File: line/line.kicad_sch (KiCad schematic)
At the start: 43 parts, among them J1 MAINS, J2 PWM, Q1 WMM38N60C2, Q2 WMM38N60C2, U1 LM324, U2 LTV-817S

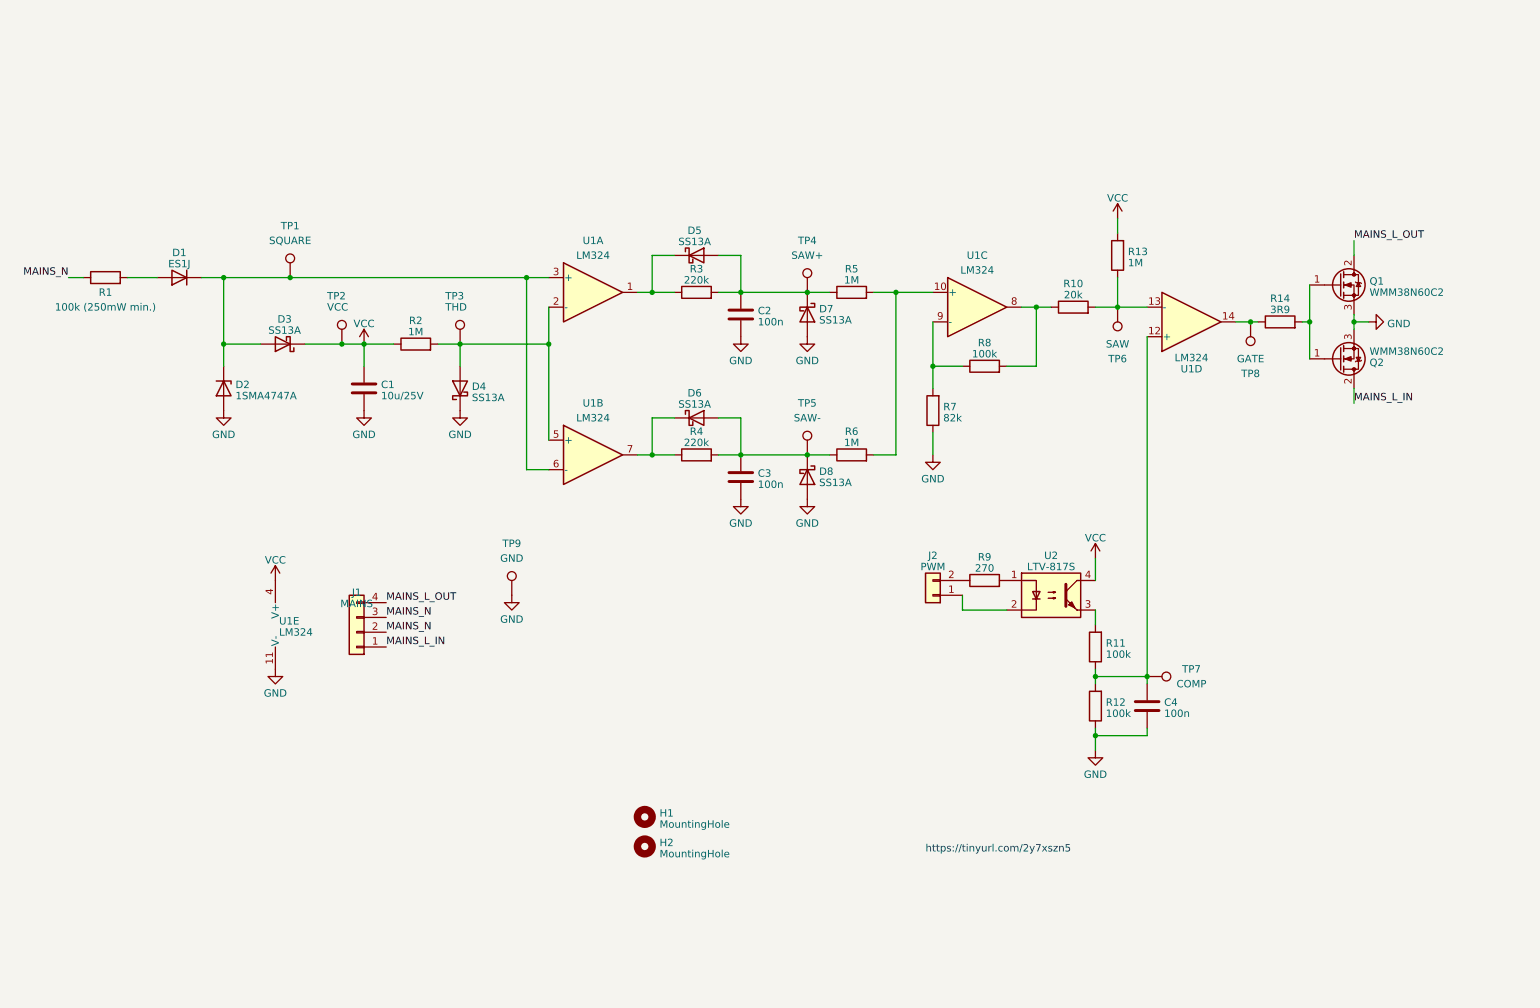
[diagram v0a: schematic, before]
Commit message: WIP
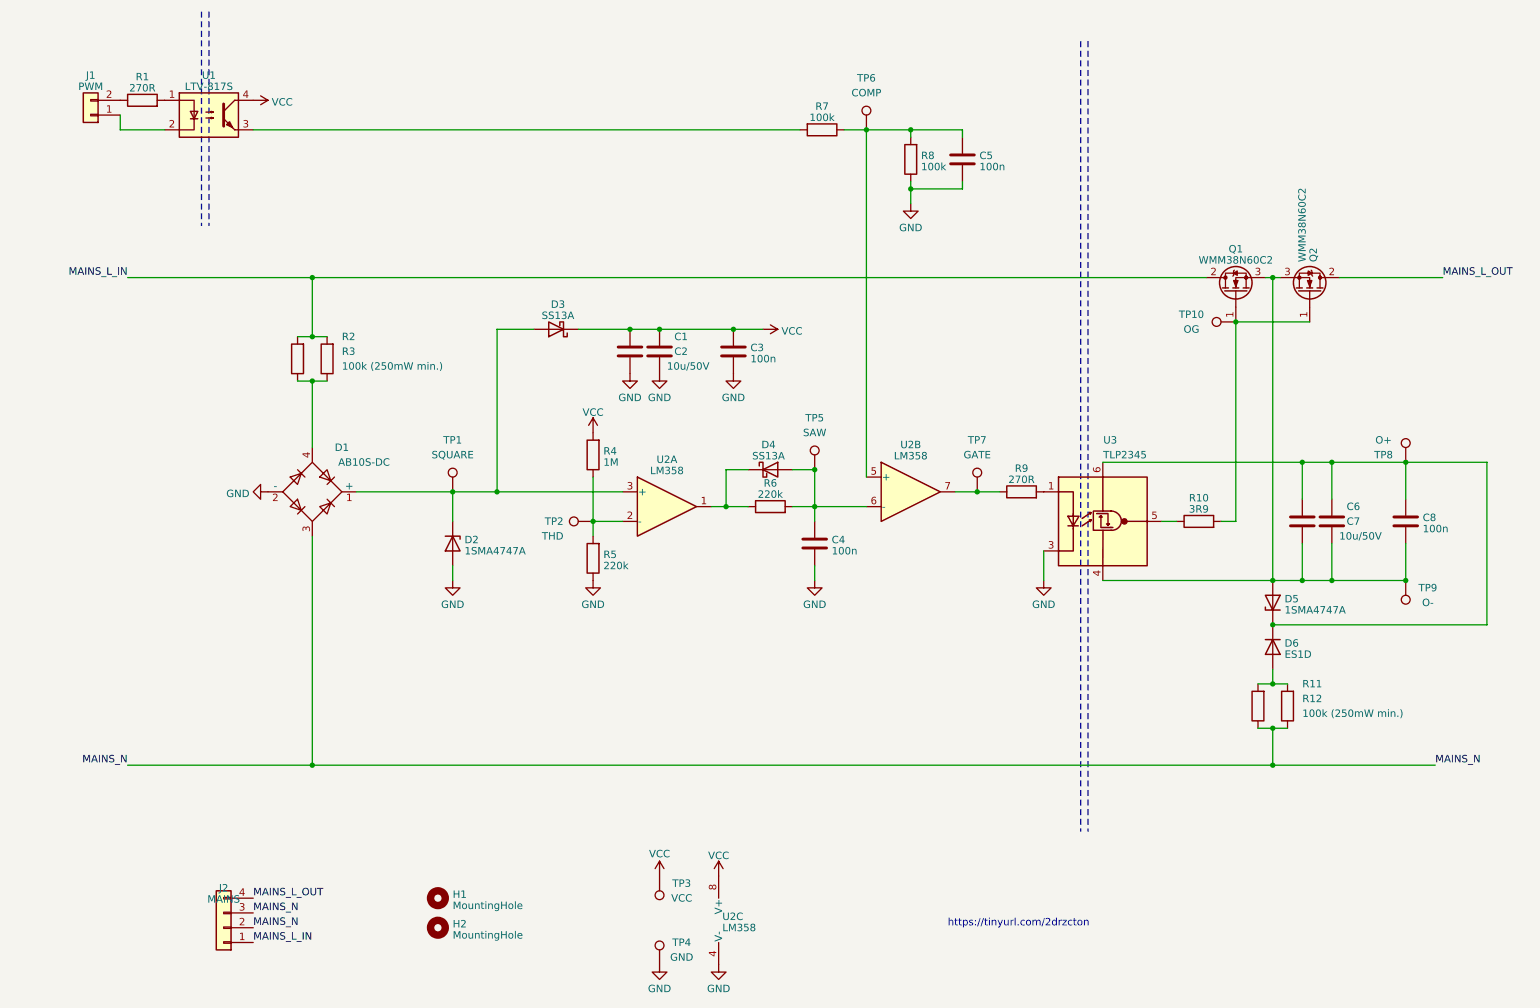
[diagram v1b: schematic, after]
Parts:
- removed D1: ES1J, Diode_SMD:D_SMA_Handsoldering, symbol Device:D
- removed D4, D6, D7, D8: SS13A, Diode_SMD:D_SMA_Handsoldering, symbol Device:D_Schottky
- removed R1: 100k (250mW min.), Resistor_SMD:R_1206_3216Metric_Pad1.30x1.75mm_HandSolder, symbol Device:R
- removed R10: 20k, Resistor_SMD:R_0805_2012Metric_Pad1.20x1.40mm_HandSolder, symbol Device:R
- removed R13, R6: 1M, Resistor_SMD:R_0805_2012Metric_Pad1.20x1.40mm_HandSolder, symbol Device:R
- removed R4: 220k, Resistor_SMD:R_0805_2012Metric_Pad1.20x1.40mm_HandSolder, symbol Device:R
- removed R7: 82k, Resistor_SMD:R_0805_2012Metric_Pad1.20x1.40mm_HandSolder, symbol Device:R
- removed R8: 100k, Resistor_SMD:R_0805_2012Metric_Pad1.20x1.40mm_HandSolder, symbol Device:R
- removed TP4: SAW+, TestPoint:TestPoint_Pad_D2.0mm, symbol Connector:TestPoint
- removed TP5: SAW-, TestPoint:TestPoint_Pad_D2.0mm, symbol Connector:TestPoint
- removed U1: LM324, Package_SO:SOIC-14_3.9x8.7mm_P1.27mm, symbol Amplifier_Operational:LM324
- added C2, C6, C7: 10u/50V, Capacitor_SMD:C_1206_3216Metric_Pad1.33x1.80mm_HandSolder, symbol Device:C
- added C8: 100n, Capacitor_SMD:C_0805_2012Metric_Pad1.18x1.45mm_HandSolder, symbol Device:C
- added D1: AB10S-DC, Diode_SMD:Diode_Bridge_Diotec_ABS, symbol Diode_Bridge:ABS10
- added D5: 1SMA4747A, Diode_SMD:D_SMA, symbol Device:D_Zener
- added D6: ES1D, Diode_SMD:D_SMA, symbol Diode:US1D
- added R11, R12, R2, R3: 100k (250mW min.), Resistor_SMD:R_1206_3216Metric_Pad1.30x1.75mm_HandSolder, symbol Device:R
- added R9: 270R, Resistor_SMD:R_0805_2012Metric_Pad1.20x1.40mm_HandSolder, symbol Device:R
- added TP10: OG, TestPoint:TestPoint_Pad_D2.0mm, symbol Connector:TestPoint
- added TP8: O+, TestPoint:TestPoint_Pad_D2.0mm, symbol Connector:TestPoint
- added TP9: O-, TestPoint:TestPoint_Pad_D2.0mm, symbol Connector:TestPoint
- added U2: LM358, Package_SO:SOIC-8_3.9x4.9mm_P1.27mm, symbol Amplifier_Operational:LM358
- added U3: TLP2345, Package_SO:SO-6L_10x3.84mm_P1.27mm, symbol Isolator:TLP2761
- C1: value 10u/25V -> 10u/50V; footprint Capacitor_SMD:C_0805_2012Metric_Pad1.18x1.45mm_HandSolder -> Capacitor_SMD:C_1206_3216Metric_Pad1.33x1.80mm_HandSolder
- D2, D3: footprint Diode_SMD:D_SMA_Handsoldering -> Diode_SMD:D_SMA
- D4: renamed from D5; footprint Diode_SMD:D_SMA_Handsoldering -> Diode_SMD:D_SMA
- R1: renamed from R9; value 270 -> 270R
- R5: value 1M -> 220k
- renumbered C2 to C4, C4 to C5, J2 to J1, J1 to J2, R14 to R10, R2 to R4, R3 to R6, R11 to R7, R12 to R8, TP3 to TP2, TP2 to TP3, TP9 to TP4, TP6 to TP5, TP7 to TP6, TP8 to TP7, U2 to U1
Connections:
- net GND: now also R5.1, C2.2, D1.2 (-), U2.4 (V-), U3.3 (K); no longer Q1.3 (S), Q2.3 (S)
- net MAINS_L_IN: now also Q1.2 (D), R2.2, R3.2; no longer Q2.2 (D)
- net MAINS_L_OUT: now also Q2.2 (D); no longer Q1.2 (D)
- net MAINS_N: now also D1.3, R11.1, R12.1
- net VCC: now also C3.1, R4.2, C2.1, U2.8 (V+); no longer R4.1
- net at D4.1 (K), R6.1: now also U2.1
- net at C4.1, D4.2 (A), R6.2: now also TP5.1, U2.6 (-); no longer R5.1
- net at TP2.1: now also R4.1, R5.2, U2.2 (-); no longer R4.2
- net at R10.1: now also U3.5 (VO); no longer TP7.1
- net at Q1.1 (G), Q2.1 (G), R10.2: now also TP10.1
- net at D2.1 (K), D3.2 (A), TP1.1: now also D1.1 (+), U2.3 (+)
- net at C5.1, R7.1, R8.2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: now also U2.5 (+)
- new net: C6.1, C7.1, C8.1, D5.1 (K), D6.1 (K), TP8.1, U3.6 (VDD)
- new net: C6.2, C7.2, C8.2, D5.2 (A), Q1.3 (S), Q2.3 (S), TP9.1, U3.4 (GND)
- new net: D1.4, R2.1, R3.1
- new net: D6.2 (A), R11.2, R12.2
- new net: R9.1, TP7.1, U2.7
- new net: R9.2, U3.1 (A)
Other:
- note added: "https://tinyurl.com/2drzcton"
- note removed: "https://tinyurl.com/2y7xszn5"
- moved on the sheet: C4, C5, D2, D4, H1, H2, J1, J2, Q1, Q2, R1, R10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
